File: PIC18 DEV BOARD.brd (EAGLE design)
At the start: 74 x 72.1 mm, 23 parts, among them IC2 7805TV, J2 J5MM, J5 J10MM, X1 22-23-2081, X3 22-23-2021, X4 22-23-2041

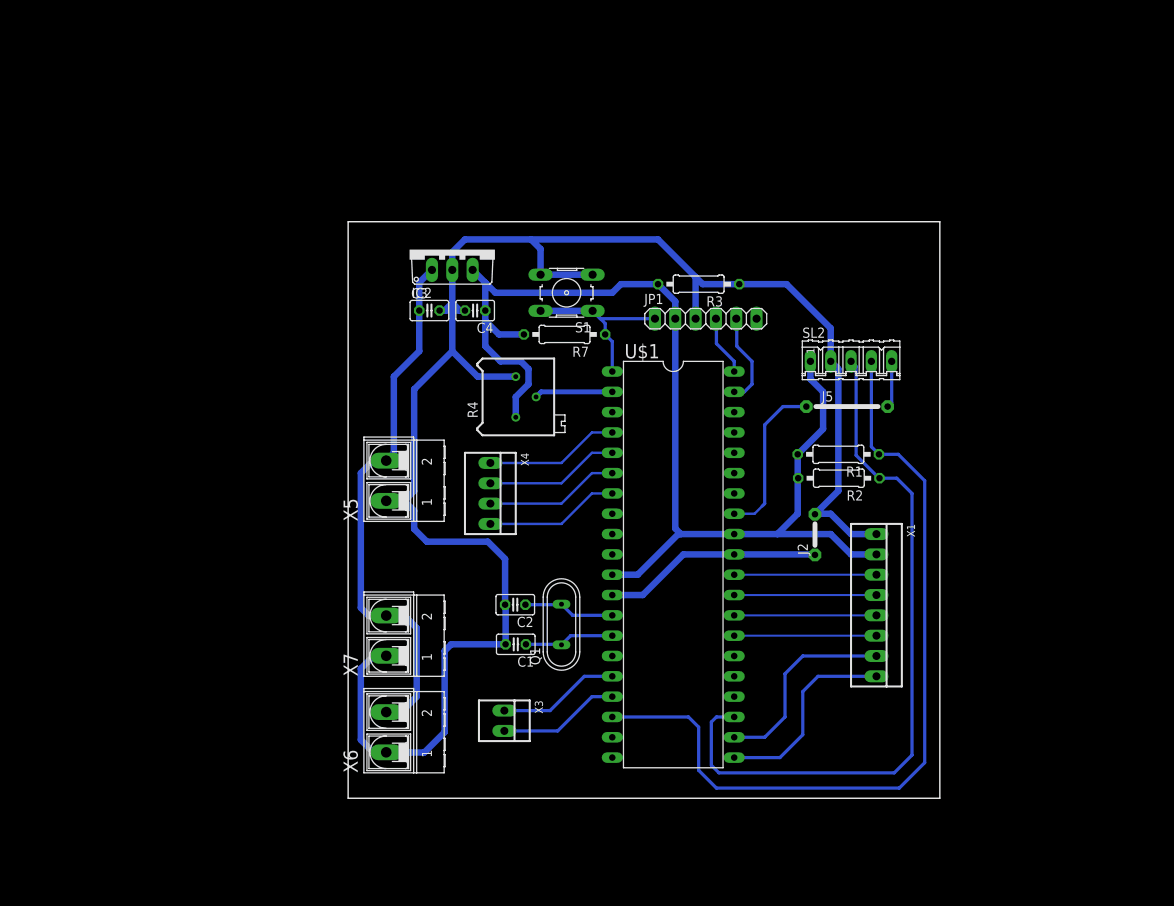
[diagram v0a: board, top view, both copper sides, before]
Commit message: Add files via upload
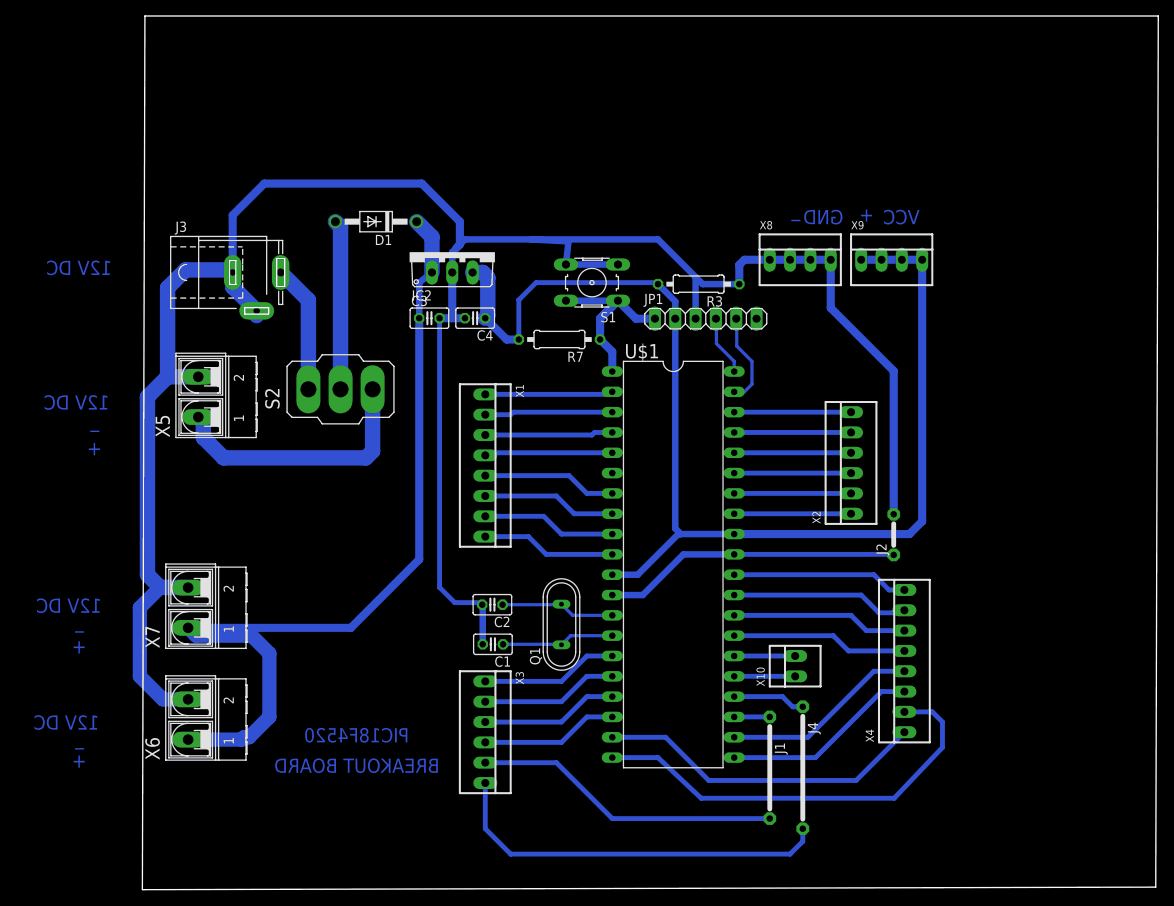
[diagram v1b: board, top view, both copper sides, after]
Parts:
- removed J5: J10MM, jumper:10
- removed R1, R2: (no value), rcl:0207/10
- removed R4: (no value), rcl:RTRIM64P
- removed SL2: (no value), con-amp-quick:05P
- added D1: 1N4004, diode:DO41-10
- added J1: J12MM, jumper:12
- added J3: 9V DC IN, con-jack:SPC4077
- added J4: J15MM, jumper:15
- added S2: P/SEL, switch:320-916
- added X10: 22-23-2021, con-molex:22-23-2021
- added X2: (no value), con-molex:22-23-2061
- added X8, X9: 22-23-2041, con-molex:22-23-2041
- X3: value 22-23-2021 -> (none); device con-molex:22-23-2021 -> con-molex:22-23-2061
- X4: value 22-23-2041 -> 22-23-2081; device con-molex:22-23-2041 -> con-molex:22-23-2081
- moved X4 55.8 mm to (69.5, 17.1), turned to 90 degrees
- moved X1 51.9 mm to (17.1, 41.6)
- moved X5 25.7 mm to (-18.7, 50.2)
- moved X7 25.0 mm to (-20.0, 23.8)
- moved X6 24.8 mm to (-20.0, 9.84)
- moved J2 9.84 mm to (68.2, 33.0)
- moved S1 3.42 mm to (30.5, 64.5)
- moved C2 2.86 mm to (18.0, 24.2)
- moved C1 2.86 mm to (18.1, 19.2)
- moved X3 2.78 mm to (17.1, 8.26)
- moved C3 0.95 mm to (10.2, 60.0)
- moved C4 0.95 mm to (15.9, 60.0)
- moved R7 0.90 mm to (26.4, 57.3)
- moved IC2 0.32 mm to (13.0, 68.3)
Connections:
- removed net N$1 (its old number): U$1.17, X3.2
- removed net N$19: C4.1, IC2.3, JP1.2, R1.2, R2.2, R3.2, R4.1, R7.2, SL2.1, U$1.11, U$1.32, X1.2
- new net N$10: U$1.36, X2.4
- new net N$17: J1.1, U$1.23
- new net N$18: J4.1, U$1.24
- new net N$20: U$1.25, X10.1
- new net N$24: U$1.26, X10.2
- new net N$26: U$1.20, X4.2
- new net N$27: U$1.21, X4.3
- new net N$29: J1.2, X3.5
- new net N$32: U$1.27, X4.5
- new net N$33: U$1.28, X4.6
- new net N$34: U$1.29, X4.7
- new net N$37: U$1.9, X1.7
- new net N$39: U$1.10, X1.8
- new net N$41: U$1.5, X1.4
- new net N$42: J4.2, X3.6
- new net N$43: D1.A, S2.2
- new net N$44: C3.1, D1.C, IC2.1, X6.1, X7.1
- new net N$45: S2.3, X5.1
- new net N$47: C4.1, IC2.3, JP1.2, R3.2, R7.2, U$1.11, U$1.32, X9.1, X9.2, X9.3, X9.4
- new net N$9: U$1.35, X2.3
- net GND: now also J3.1, J3.2, X5.2, X6.2, X7.2, X8.1, X8.2, X8.3, X8.4; no longer R4.3, SL2.2, X1.1, X5.1, X6.1, X7.1
- net N$11: now also U$1.37, X2.5; no longer J5.1, U$1.33
- net N$12: now also U$1.38, X2.6; no longer U$1.16, X3.1
- net N$13: now also U$1.15, X3.1; no longer U$1.4, X4.1
- net N$14: now also U$1.16, X3.2; no longer U$1.5, X4.2
- net N$15: now also U$1.17, X3.3; no longer U$1.6, X4.3
- net N$16: now also U$1.18, X3.4; no longer U$1.7, X4.4
- net N$2: now also U$1.2, X1.1; no longer U$1.30, X1.3
- net N$25: now also U$1.19, X4.1; no longer R4.2, U$1.2
- net N$28: now also U$1.22, X4.4; no longer C3.1, IC2.1, X5.2, X6.2, X7.2
- net N$3: now also U$1.3, X1.2; no longer U$1.29, X1.4
- net N$35: now also U$1.30, X4.8; no longer R1.1, SL2.4, U$1.18
- net N$36: now also U$1.8, X1.6; no longer R2.1, SL2.3, U$1.23
- net N$4: now also U$1.4, X1.3; no longer U$1.28, X1.5
- net N$5: now also J3.3, S2.1; no longer U$1.27, X1.6
- net N$6: now also U$1.7, X1.5; no longer U$1.22, X1.7
- net N$7: now also U$1.33, X2.1; no longer U$1.21, X1.8
- net N$8: now also U$1.34, X2.2; no longer J5.2, SL2.5
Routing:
- net N$47: track 0.00 -> 150.2 mm
- net N$19: track 144.8 -> 0.00 mm
- net N$44: track 0.00 -> 107.0 mm
- net N$35: track 101.6 -> 22.1 mm
- net N$36: track 88.6 -> 16.8 mm
- net GND: track 223.5 -> 291.2 mm
- net N$26: track 0.00 -> 54.5 mm
- net N$42: track 0.00 -> 49.0 mm
- net N$28: track 68.1 -> 24.7 mm
- net N$29: track 0.00 -> 38.5 mm
- net N$45: track 0.00 -> 33.1 mm
- net N$25: track 9.79 -> 41.9 mm
- net N$27: track 0.00 -> 24.7 mm
- net N$34: track 0.00 -> 23.6 mm
- net N$43: track 0.00 -> 22.6 mm
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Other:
- board size 74 x 72.1 mm -> 127 x 109.2 mm
- board text added: "+"
- board text added: "12V DC"
- board text added: "BREAKOUT BOARD"
- board text added: "GND"
- board text added: "PIC18F4520"
- board text added: "VCC"
- board text added: "_"
